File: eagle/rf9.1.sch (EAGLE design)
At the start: 104 parts, among them U1 MIC5219 3.6V

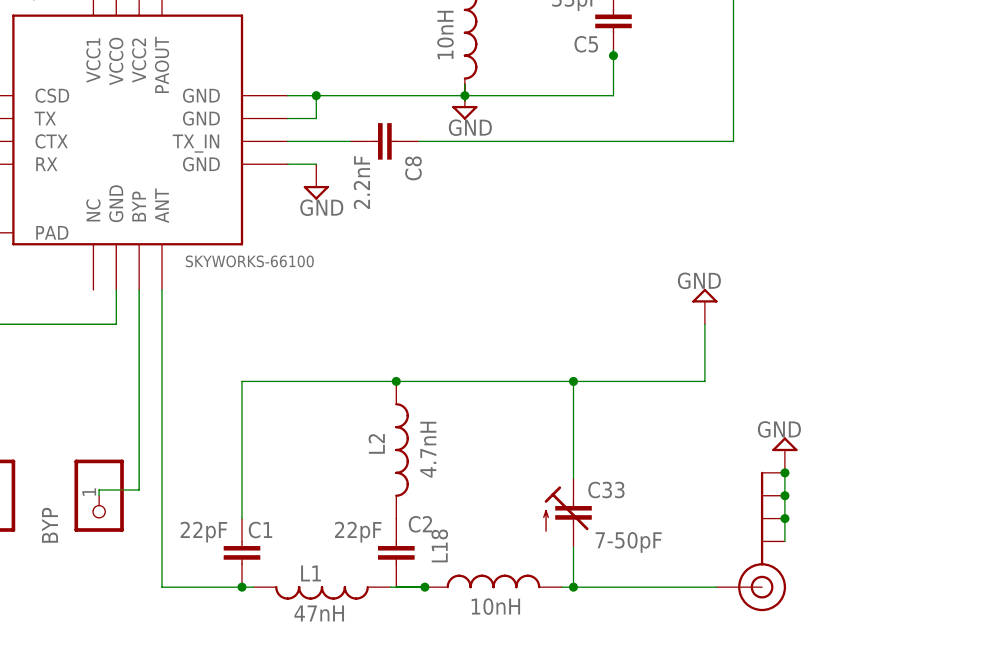
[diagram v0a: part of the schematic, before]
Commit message: Build settings, Eagle files
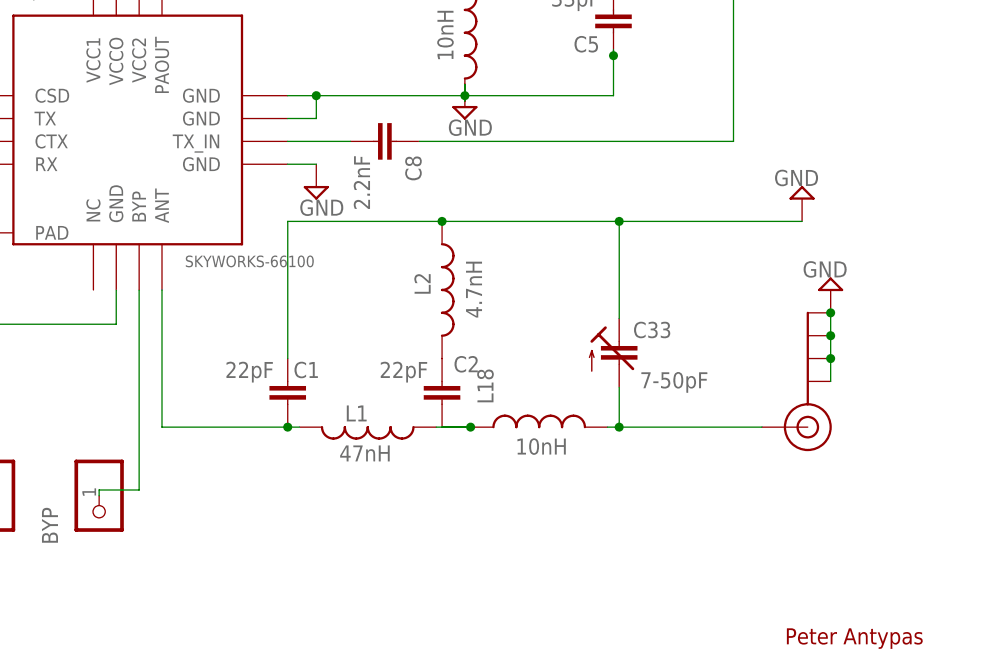
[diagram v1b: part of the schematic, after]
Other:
- note added: "Peter Antypas"
- moved on the sheet: C1, C2, C33, L1, L18, L2
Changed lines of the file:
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@@
 <part name="C41" library="SparkFun-Capacitors" deviceset="CAP" device="0603-CAP" value="20pF"/>
 <part name="SUPPLY5" library="supply2" deviceset="GND" device=""/>
+<part name="FRAME1" library="SparkFun-Retired" deviceset="FRAME-A3" device=""/>
 </parts>
 <sheets>
 <sheet>
 <plain>
+<text x="133.35" y="-149.86" size="1.778" layer="94">Peter Antypas</text>
 </plain>
 <instances>
@@
 <instance part="C22" gate="G$1" x="-97.155" y="15.24"/>
 <instance part="SUPPLY19" gate="GND" x="-100.965" y="10.16"/>
-<instance part="SUPPLY20" gate="GND" x="133.35" y="-128.27" rot="R180"/>
+<instance part="SUPPLY20" gate="GND" x="138.43" y="-110.49" rot="R180"/>
 <instance part="C31" gate="G$1" x="-16.51" y="50.165"/>
 <instance part="L3" gate="G$1" x="7.62" y="33.02" smashed="yes">
@@
 <instance part="VCC1" gate="G$1" x="6.35" y="94.615" rot="R90"/>
 <instance part="SUPPLY1" gate="G$1" x="13.97" y="97.155"/>
-<instance part="J$1" gate="1" x="130.81" y="-143.51" rot="R180"/>
+<instance part="J$1" gate="1" x="135.89" y="-125.73" rot="R180"/>
 <instance part="U$3" gate="G$1" x="-125.095" y="-81.28" rot="R180"/>
 <instance part="SUPPLY24" gate="GND" x="-125.095" y="-111.76"/>
@@
 <instance part="GND@2" gate="G$1" x="-55.245" y="-95.25" rot="R90"/>
 <instance part="SUPPLY18" gate="GND" x="-55.245" y="-109.22"/>
-<instance part="SUPPLY2" gate="GND" x="124.46" y="-111.76" rot="R180"/>
+<instance part="SUPPLY2" gate="GND" x="135.255" y="-100.33" rot="R180"/>
 <instance part="SUPPLY14" gate="GND" x="14.605" y="-106.68"/>
 <instance part="SUPPLY15" gate="GND" x="81.28" y="-99.06"/>
 <instance part="SUPPLY21" gate="GND" x="97.79" y="-90.17"/>
-<instance part="L1" gate="G$1" x="81.915" y="-143.51" smashed="yes" rot="R270">
-<attribute name="NAME" x="79.375" y="-142.875" size="1.778" layer="95"/>
-<attribute name="VALUE" x="78.74" y="-147.32" size="1.778" layer="96"/>
-</instance>
-<instance part="L2" gate="G$1" x="90.17" y="-128.27" smashed="yes">
-<attribute name="NAME" x="88.9" y="-128.905" size="1.778" layer="95" rot="R90"/>
-<attribute name="VALUE" x="94.615" y="-131.445" size="1.778" layer="96" rot="R90"/>
-</instance>
-<instance part="C1" gate="G$1" x="73.025" y="-138.43" smashed="yes" rot="R180">
-<attribute name="NAME" x="76.581" y="-136.271" size="1.778" layer="95" rot="R180"/>
-<attribute name="VALUE" x="71.501" y="-136.271" size="1.778" layer="96" rot="R180"/>
-</instance>
-<instance part="C2" gate="G$1" x="90.17" y="-138.43" smashed="yes" rot="R180">
-<attribute name="NAME" x="94.361" y="-135.636" size="1.778" layer="95" rot="R180"/>
-<attribute name="VALUE" x="88.646" y="-136.271" size="1.778" layer="96" rot="R180"/>
+<instance part="L1" gate="G$1" x="86.995" y="-125.73" smashed="yes" rot="R270">
+<attribute name="NAME" x="84.455" y="-125.095" size="1.778" layer="95"/>
+<attribute name="VALUE" x="83.82" y="-129.54" size="1.778" layer="96"/>
+</instance>
+<instance part="L2" gate="G$1" x="95.25" y="-110.49" smashed="yes">
+<attribute name="NAME" x="93.98" y="-111.125" size="1.778" layer="95" rot="R90"/>
+<attribute name="VALUE" x="99.695" y="-113.665" size="1.778" layer="96" rot="R90"/>
+</instance>
+<instance part="C1" gate="G$1" x="78.105" y="-120.65" smashed="yes" rot="R180">
+<attribute name="NAME" x="81.661" y="-118.491" size="1.778" layer="95" rot="R180"/>
+<attribute name="VALUE" x="76.581" y="-118.491" size="1.778" layer="96" rot="R180"/>
+</instance>
+<instance part="C2" gate="G$1" x="95.25" y="-120.65" smashed="yes" rot="R180">
+<attribute name="NAME" x="99.441" y="-117.856" size="1.778" layer="95" rot="R180"/>
+<attribute name="VALUE" x="93.726" y="-118.491" size="1.778" layer="96" rot="R180"/>
 </instance>
 <instance part="C5" gate="G$1" x="114.3" y="-79.375" smashed="yes" rot="R180">
@@
 <instance part="R1" gate="G$1" x="7.62" y="12.7" rot="R90"/>
 <instance part="L24" gate="G$1" x="0" y="55.88" rot="R90"/>
-<instance part="L18" gate="G$1" x="100.965" y="-143.51" smashed="yes" rot="R90">
-<attribute name="NAME" x="95.885" y="-140.97" size="1.778" layer="95" rot="R90"/>
-<attribute name="VALUE" x="104.14" y="-144.78" size="1.778" layer="96" rot="R180"/>
-</instance>
-<instance part="C33" gate="G$1" x="109.855" y="-133.985"/>
+<instance part="L18" gate="G$1" x="106.045" y="-125.73" smashed="yes" rot="R90">
+<attribute name="NAME" x="100.965" y="-123.19" size="1.778" layer="95" rot="R90"/>
+<attribute name="VALUE" x="109.22" y="-127" size="1.778" layer="96" rot="R180"/>
+</instance>
+<instance part="C33" gate="G$1" x="114.935" y="-116.205"/>
 <instance part="L25" gate="G$1" x="26.67" y="-24.765" rot="R90"/>
 <instance part="C32" gate="G$1" x="17.78" y="-29.845"/>
@@
 <instance part="C41" gate="G$1" x="-102.235" y="-15.24" rot="R180"/>
 <instance part="SUPPLY5" gate="GND" x="-102.235" y="-25.4"/>
+<instance part="FRAME1" gate="G$1" x="-196.215" y="-154.305"/>
 </instances>
 <busses>
@@
 <pinref part="SUPPLY20" gate="GND" pin="GND"/>
 <pinref part="J$1" gate="1" pin="GND@2"/>
-<wire x1="133.35" y1="-133.35" x2="133.35" y2="-130.81" width="0.1524" layer="91"/>
-<junction x="133.35" y="-130.81"/>
+<wire x1="138.43" y1="-115.57" x2="138.43" y2="-113.03" width="0.1524" layer="91"/>
+<junction x="138.43" y="-113.03"/>
 <pinref part="J$1" gate="1" pin="GND@1"/>
-<wire x1="133.35" y1="-135.89" x2="133.35" y2="-133.35" width="0.1524" layer="91"/>
-<junction x="133.35" y="-133.35"/>
+<wire x1="138.43" y1="-118.11" x2="138.43" y2="-115.57" width="0.1524" layer="91"/>
+<junction x="138.43" y="-115.57"/>
 <pinref part="J$1" gate="1" pin="GND@0"/>
-<wire x1="133.35" y1="-138.43" x2="133.35" y2="-135.89" width="0.1524" layer="91"/>
-<junction x="133.35" y="-135.89"/>
+<wire x1="138.43" y1="-120.65" x2="138.43" y2="-118.11" width="0.1524" layer="91"/>
+<junction x="138.43" y="-118.11"/>
 </segment>
 <segment>
@@
 <pinref part="SUPPLY2" gate="GND" pin="GND"/>
 <pinref part="L2" gate="G$1" pin="1"/>
-<wire x1="124.46" y1="-120.65" x2="124.46" y2="-114.3" width="0.1524" layer="91"/>
 <pinref part="C1" gate="G$1" pin="2"/>
-<wire x1="90.17" y1="-120.65" x2="109.855" y2="-120.65" width="0.1524" layer="91"/>
-<wire x1="109.855" y1="-120.65" x2="124.46" y2="-120.65" width="0.1524" layer="91"/>
-<wire x1="73.025" y1="-135.89" x2="73.025" y2="-120.65" width="0.1524" layer="91"/>
-<wire x1="73.025" y1="-120.65" x2="90.17" y2="-120.65" width="0.1524" layer="91"/>
-<junction x="90.17" y="-120.65"/>
-<wire x1="109.855" y1="-131.445" x2="109.855" y2="-120.65" width="0.1524" layer="91"/>
-<junction x="109.855" y="-120.65"/>
+<wire x1="95.25" y1="-102.87" x2="114.935" y2="-102.87" width="0.1524" layer="91"/>
+<wire x1="114.935" y1="-102.87" x2="135.255" y2="-102.87" width="0.1524" layer="91"/>
+<wire x1="78.105" y1="-118.11" x2="78.105" y2="-102.87" width="0.1524" layer="91"/>
+<wire x1="78.105" y1="-102.87" x2="95.25" y2="-102.87" width="0.1524" layer="91"/>
+<junction x="95.25" y="-102.87"/>
+<wire x1="114.935" y1="-113.665" x2="114.935" y2="-102.87" width="0.1524" layer="91"/>
+<junction x="114.935" y="-102.87"/>
 <pinref part="C33" gate="G$1" pin="E"/>
 </segment>
@@
 <pinref part="L1" gate="G$1" pin="1"/>
 <pinref part="C2" gate="G$1" pin="1"/>
-<wire x1="90.17" y1="-143.51" x2="93.345" y2="-143.51" width="0.1524" layer="91"/>
+<wire x1="95.25" y1="-125.73" x2="98.425" y2="-125.73" width="0.1524" layer="91"/>
 <pinref part="L18" gate="G$1" pin="1"/>
-<junction x="93.345" y="-143.51"/>
-<wire x1="93.345" y1="-143.51" x2="89.535" y2="-143.51" width="0.1524" layer="91"/>
+<junction x="98.425" y="-125.73"/>
+<wire x1="98.425" y1="-125.73" x2="94.615" y2="-125.73" width="0.1524" layer="91"/>
 </segment>
 </net>
@@
 <pinref part="L1" gate="G$1" pin="2"/>
 <pinref part="C1" gate="G$1" pin="1"/>
-<wire x1="73.025" y1="-143.51" x2="74.295" y2="-143.51" width="0.1524" layer="91"/>
-<wire x1="73.025" y1="-143.51" x2="64.135" y2="-143.51" width="0.1524" layer="91"/>
-<wire x1="64.135" y1="-143.51" x2="64.135" y2="-110.49" width="0.1524" layer="91"/>
-<junction x="73.025" y="-143.51"/>
+<wire x1="78.105" y1="-125.73" x2="79.375" y2="-125.73" width="0.1524" layer="91"/>
+<wire x1="78.105" y1="-125.73" x2="64.135" y2="-125.73" width="0.1524" layer="91"/>
+<wire x1="64.135" y1="-125.73" x2="64.135" y2="-110.49" width="0.1524" layer="91"/>
+<junction x="78.105" y="-125.73"/>
 <pinref part="U$4" gate="G$1" pin="ANT"/>
 </segment>
@@
 <pinref part="L18" gate="G$1" pin="2"/>
 <pinref part="J$1" gate="1" pin="SIGNAL"/>
-<wire x1="108.585" y1="-143.51" x2="109.855" y2="-143.51" width="0.1524" layer="91"/>
+<wire x1="113.665" y1="-125.73" x2="114.935" y2="-125.73" width="0.1524" layer="91"/>
 <pinref part="C33" gate="G$1" pin="A"/>
-<wire x1="109.855" y1="-143.51" x2="125.73" y2="-143.51" width="0.1524" layer="91"/>
-<wire x1="109.855" y1="-139.065" x2="109.855" y2="-143.51" width="0.1524" layer="91"/>
-<junction x="109.855" y="-143.51"/>
-</segment>
-</net>
+<wire x1="114.935" y1="-125.73" x2="130.81" y2="-125.73" width="0.1524" layer="91"/>
+<wire x1="114.935" y1="-121.285" x2="114.935" y2="-125.73" width="0.1524" layer="91"/>
+<junction x="114.935" y="-125.73"/>
+</segment>
+</net>
